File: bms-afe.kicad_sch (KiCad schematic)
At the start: 0 parts

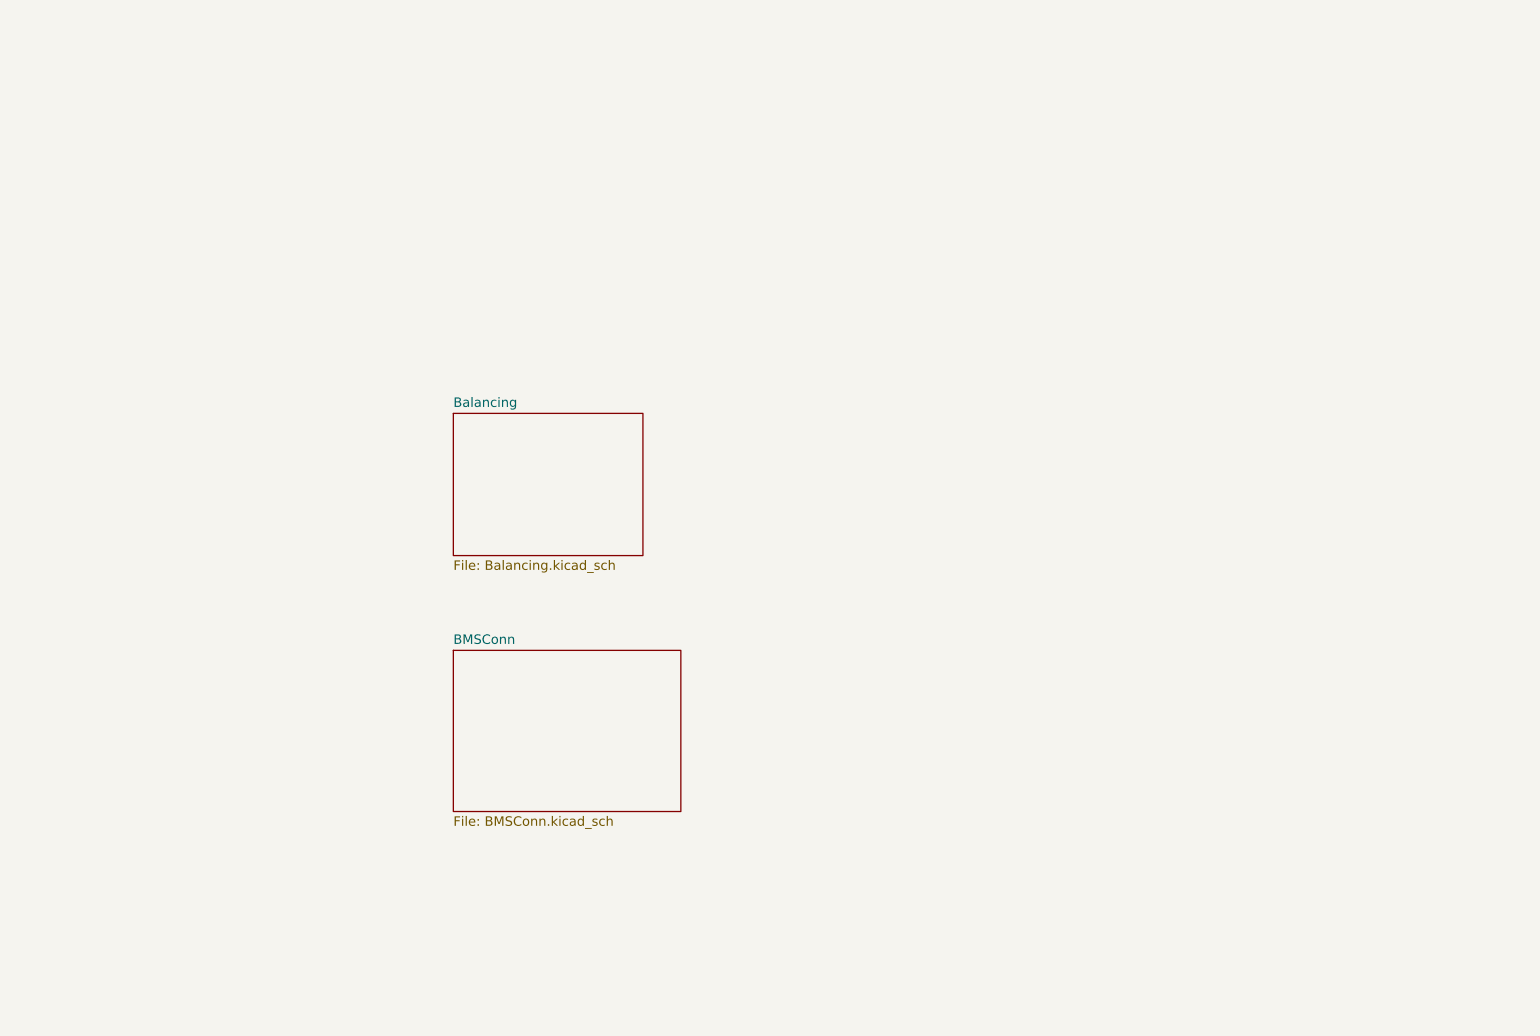
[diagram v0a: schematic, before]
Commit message: mostly done afe ic
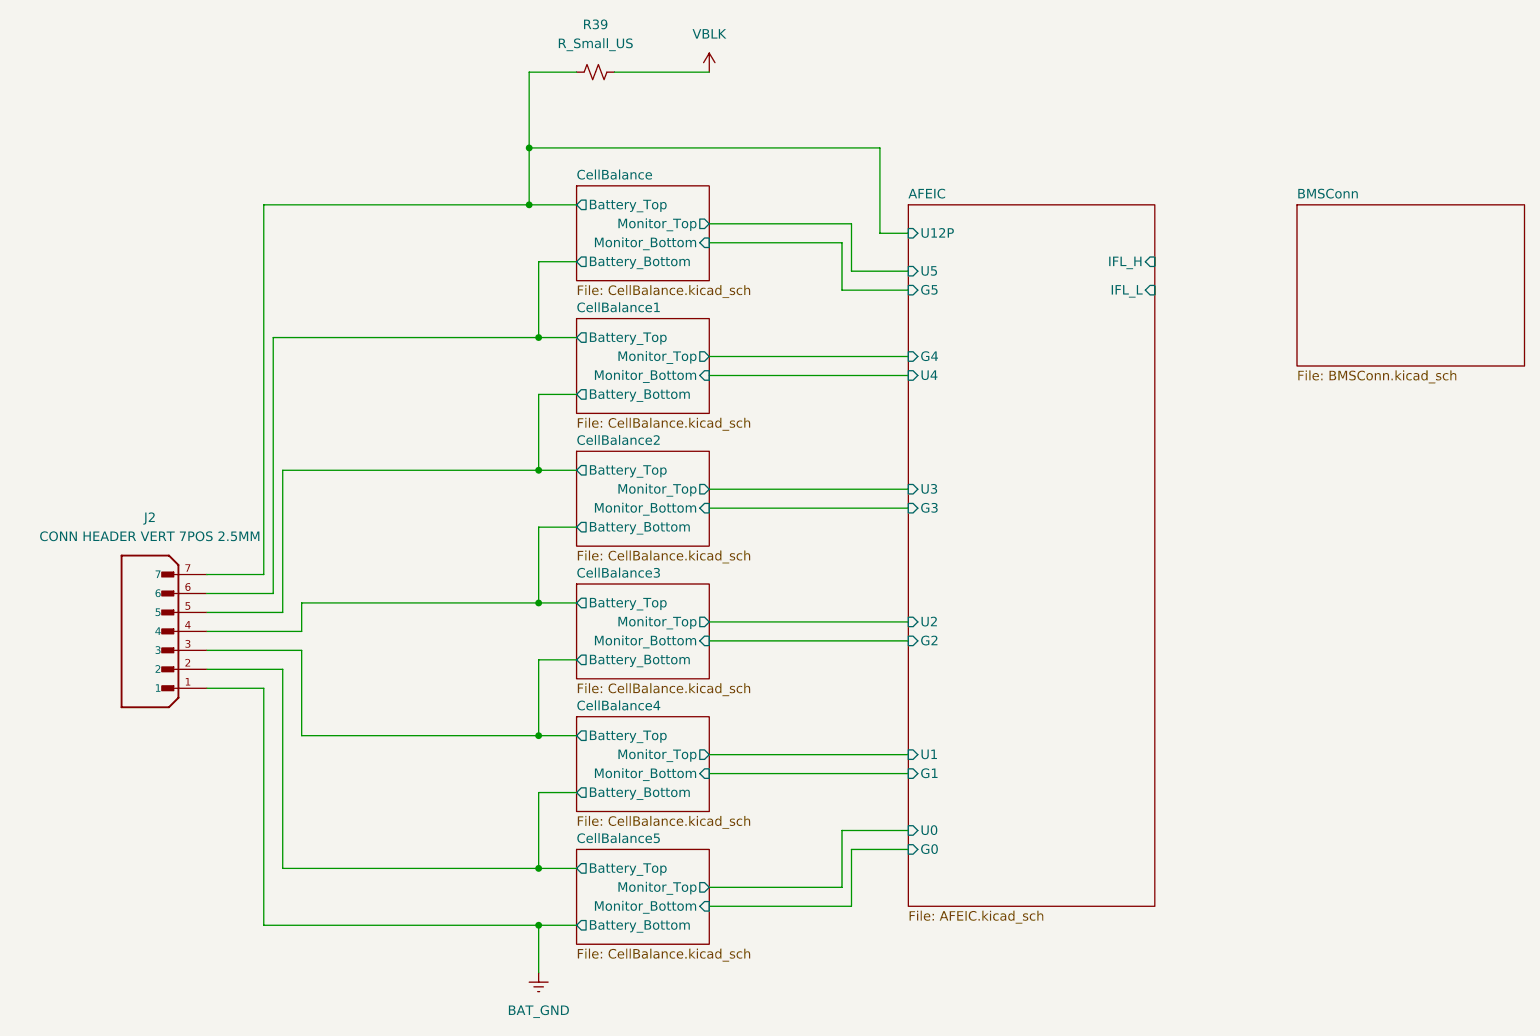
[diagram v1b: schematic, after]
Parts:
- added J2: CONN HEADER VERT 7POS 2.5MM, footprints:JST_B7B-XH-A_LF__SN_, symbol symbols:B7B-XH-A_LF__SN_
- added R39: R_Small_US, symbol Device:R_Small_US
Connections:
- new net AFEIC/U12P: J2.7, R39.1
- new net BAT_GND: J2.1
- new net CellBalance/Battery_Bottom: J2.6
- new net CellBalance1/Battery_Bottom: J2.5
- new net CellBalance2/Battery_Bottom: J2.4
- new net CellBalance3/Battery_Bottom: J2.3
- new net CellBalance4/Battery_Bottom: J2.2
- new net VBLK: R39.2
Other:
- removed sheet Balancing
- added sheet AFEIC (AFEIC.kicad_sch)
- added sheet CellBalance (CellBalance.kicad_sch)
- added sheet CellBalance1 (CellBalance.kicad_sch)
- added sheet CellBalance2 (CellBalance.kicad_sch)
- added sheet CellBalance3 (CellBalance.kicad_sch)
- added sheet CellBalance4 (CellBalance.kicad_sch)
- added sheet CellBalance5 (CellBalance.kicad_sch)
